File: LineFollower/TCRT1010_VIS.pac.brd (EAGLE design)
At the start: 12 x 35.2 mm, 10 parts, among them U1 TCRT5000, U2 LM358DR

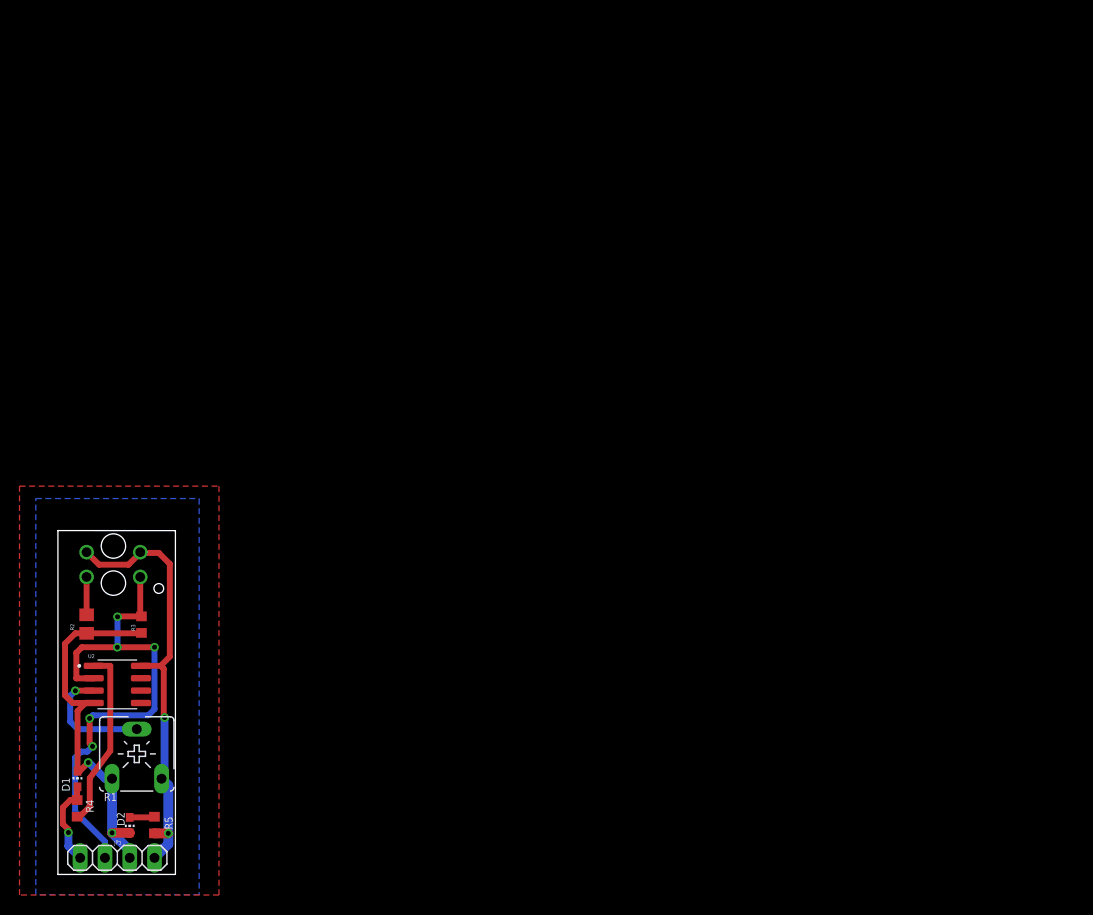
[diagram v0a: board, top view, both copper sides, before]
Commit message: 5 channel module
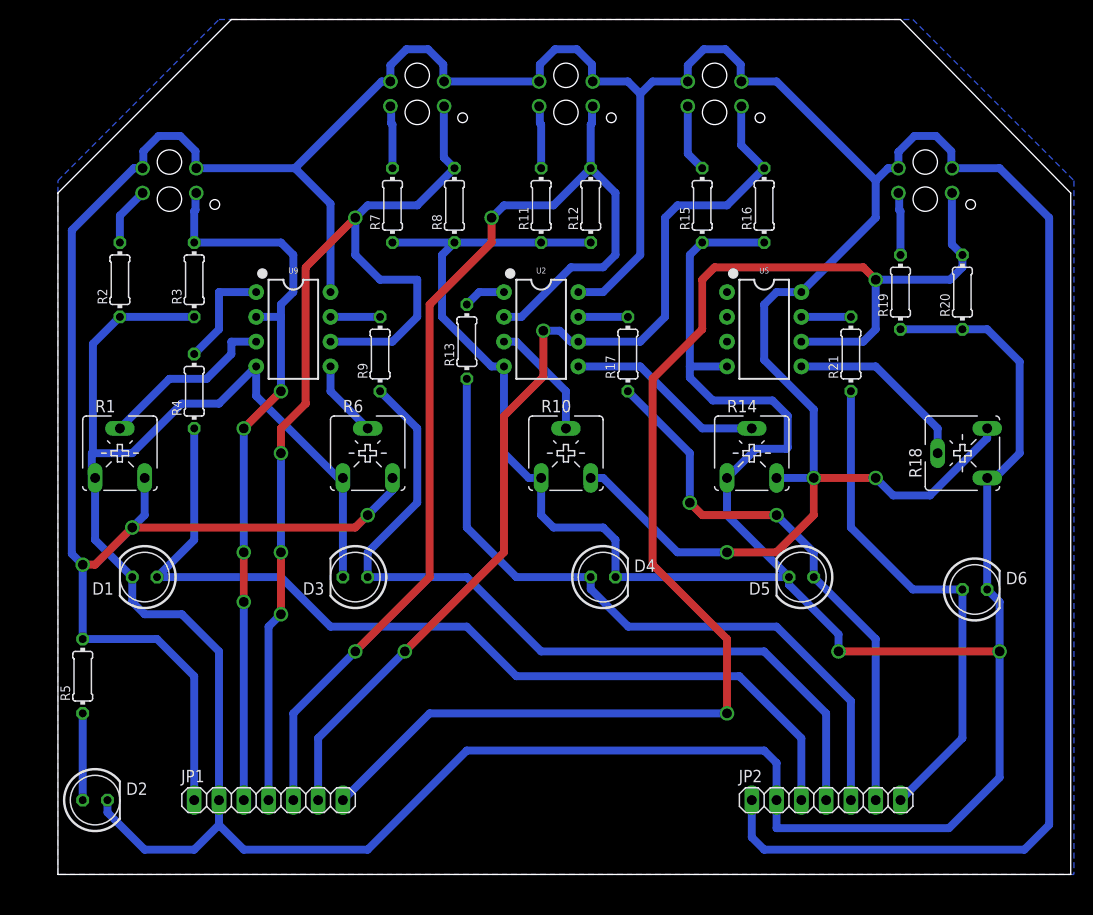
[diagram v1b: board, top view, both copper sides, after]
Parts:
- added D3, D4, D5, D6: LED5MM, MIA_LIBRARY-2-2-2:LED5MM
- added JP2: (no value), MIA_LIBRARY-2-2-2:1X07
- added R10, R14, R18, R6: (no value), MIA_LIBRARY-2-2-2:CA6V
- added R11, R15, R19, R7: 100, MIA_LIBRARY-2-2-2:0204/7
- added R12, R16, R20, R8: 10k, MIA_LIBRARY-2-2-2:0204/7
- added R13, R17, R21, R9: 330, MIA_LIBRARY-2-2-2:0204/7
- added U3, U4, U6, U7: TCRT5000, TCRT5000:OPTO_TCRT5000
- added U5, U9: LM358, MIA_LIBRARY-2-2-2:DIP08
- D1, D2: value (none) -> LED5MM; device 52101-101-REV-A_v16:LED_CHIP-LED0603MP -> MIA_LIBRARY-2-2-2:LED5MM
- JP1: device MIA_LIBRARY-2-2-2:1X04 -> MIA_LIBRARY-2-2-2:1X07
- R2: device rcl:R0805 -> MIA_LIBRARY-2-2-2:0204/7
- R3, R4, R5: device rcl:R0603 -> MIA_LIBRARY-2-2-2:0204/7
- U2: value LM358DR -> LM358; device IC:LM358DR -> MIA_LIBRARY-2-2-2:DIP08
- moved U2 56.7 mm to (49.5, 55.9), turned to 270 degrees
- moved R4 44.4 mm to (14.0, 49.5), turned to 90 degrees
- moved U1 39.8 mm to (11.4, 71.1)
- moved R3 35.8 mm to (14.0, 61.0)
- moved R2 35.5 mm to (6.35, 61.0)
- moved R1 30.9 mm to (6.35, 43.2)
- moved D1 21.8 mm to (8.89, 30.5), turned to 180 degrees
- moved R5 16.9 mm to (2.54, 20.3), turned to 90 degrees
- moved JP1 16.6 mm to (21.6, 7.62), turned to 0 degrees
- moved D2 4.38 mm to (3.81, 7.62), turned to 0 degrees
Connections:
- new net D1: D3.A, JP2.4, R9.1
- new net D2: D4.A, JP2.5, R13.1
- new net D3: D5.A, JP2.6, R17.1
- new net D4: D6.A, JP2.7, R21.1
- new net IN3+: R10.S, U2.3
- new net IN3-: JP1.5, R12.2, U2.2, U4.E
- new net IN4+: R14.S, U2.5
- new net IN4-: JP1.6, R16.2, U2.6, U6.E
- new net IN5+: U5.3
- new net IN5-: U5.2
- new net IN6+: R18.S, U5.5
- new net IN6-: JP1.7, R20.2, U5.6, U7.E
- new net N$3: R7.2, U3.CATH
- new net N$4: R11.2, U4.CATH
- new net N$5: R15.2, U6.CATH
- new net N$6: R19.2, U7.CATH
- new net OUT3: R13.2, U2.1
- new net OUT4: R17.2, U2.7
- new net OUT5: U5.1
- new net OUT6: R21.2, U5.7
- net D0: now also JP2.3; no longer JP1.4
- net GND: now also D1.K, D2.K, D3.K, D4.K, D5.K, D6.K, JP2.2, R10.A, R11.1, R12.1, R14.A, R15.1, R16.1, R18.A, R19.1, R20.1, R6.A, R7.1, R8.1, U5.4, U9.4; no longer D1.C, D2.C
- net IN1+: now also U9.3; no longer U2.3
- net IN1-: now also U9.2; no longer U2.2
- net IN2+: now also R6.S, U9.5; no longer U2.5
- net IN2-: now also JP1.4, R8.2, U3.E, U9.6; no longer U2.6
- net OUT1: now also U9.1; no longer U2.1
- net OUT2: now also R9.2, U9.7; no longer U2.7
- net VCC: now also JP2.1, R10.E, R14.E, R18.E, R6.E, U3.A, U3.COLL, U4.A, U4.COLL, U5.8, U6.A, U6.COLL, U7.A, U7.COLL, U9.8
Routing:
- net VCC: track 45.2 -> 480.4 mm, vias 2 -> 6
- net GND: track 39.8 -> 453.8 mm
- net IN6-: track 0.00 -> 142.3 mm, vias 0 -> 2
- net IN3-: track 0.00 -> 110.8 mm, vias 0 -> 2
- net IN2-: track 0.00 -> 107.4 mm, vias 0 -> 4
- net IN4-: track 0.00 -> 101.4 mm, vias 0 -> 2
- net D0: track 9.13 -> 96.0 mm, vias 1 -> 0
- net D1: track 0.00 -> 84.4 mm
- net D2: track 0.00 -> 72.9 mm
- net D3: track 0.00 -> 56.9 mm, vias 0 -> 2
- net D4: track 0.00 -> 52.3 mm
- net IN1-: track 52.5 -> 76.4 mm, vias 5 -> 4
- net IN4+: track 0.00 -> 20.4 mm
- net IN6+: track 0.00 -> 19.1 mm
- net IN3+: track 0.00 -> 12.3 mm
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- removed copper zone on layer 1, net GND
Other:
- board size 12 x 35.2 mm -> 103.8 x 87.6 mm
